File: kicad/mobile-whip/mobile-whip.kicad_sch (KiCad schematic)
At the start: 42 parts, among them J1 Conn_Coaxial, J2 USB_C_Receptacle_USB2.0, SW1 MK-12C02-G025, U1 LTC6268IS6, U2 TP4054, U3 LP2985-3.3

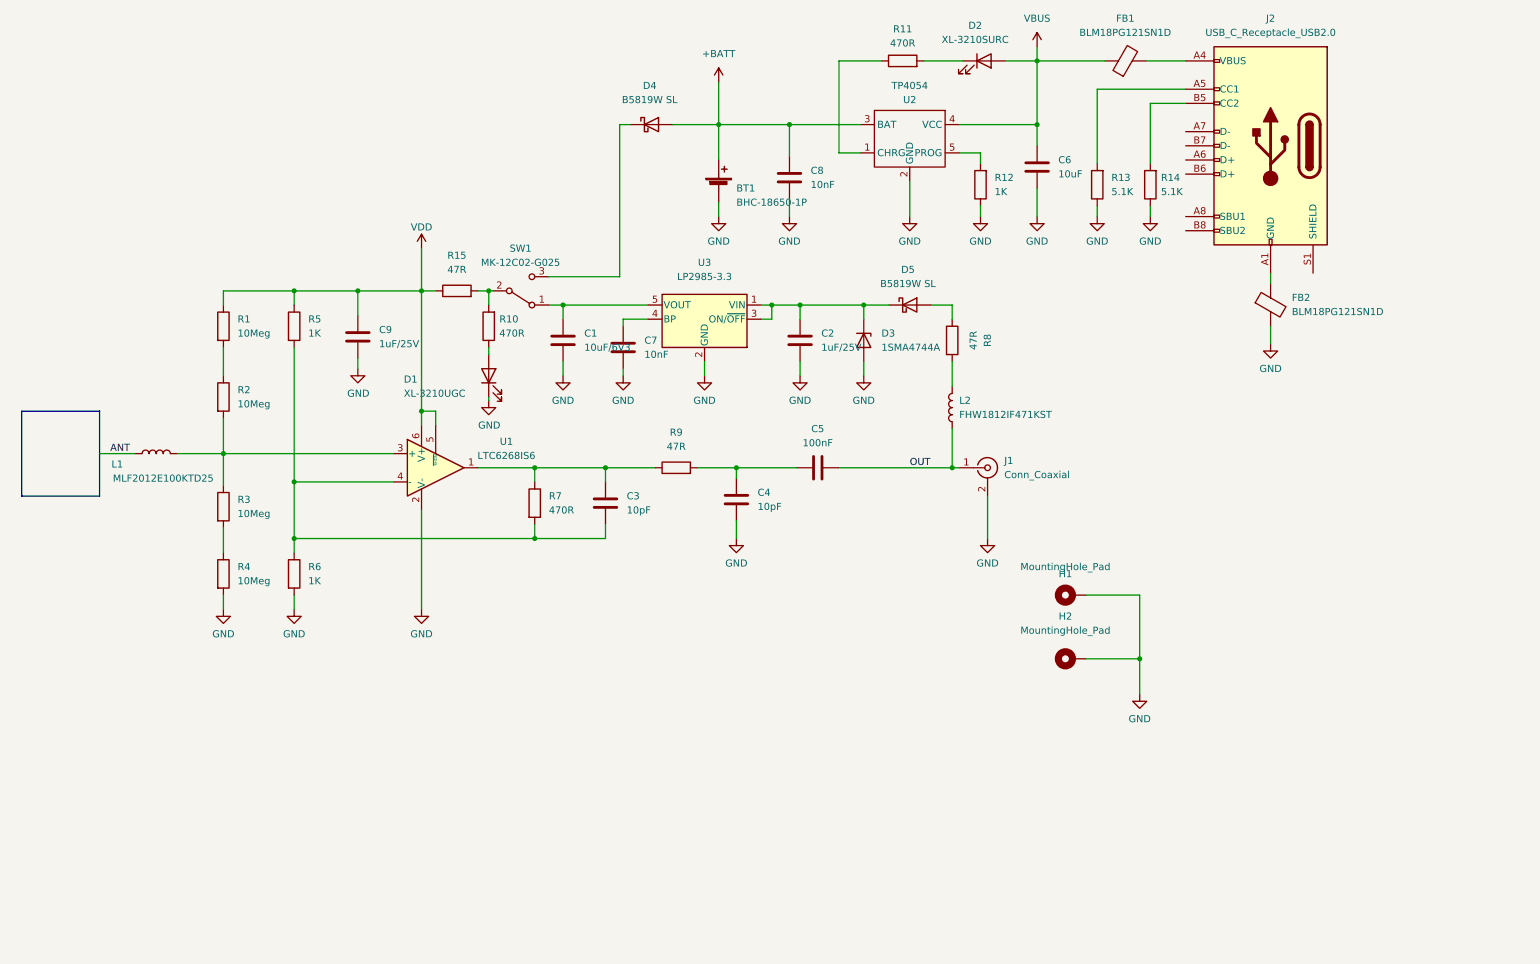
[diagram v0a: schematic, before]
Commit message: Finalize design
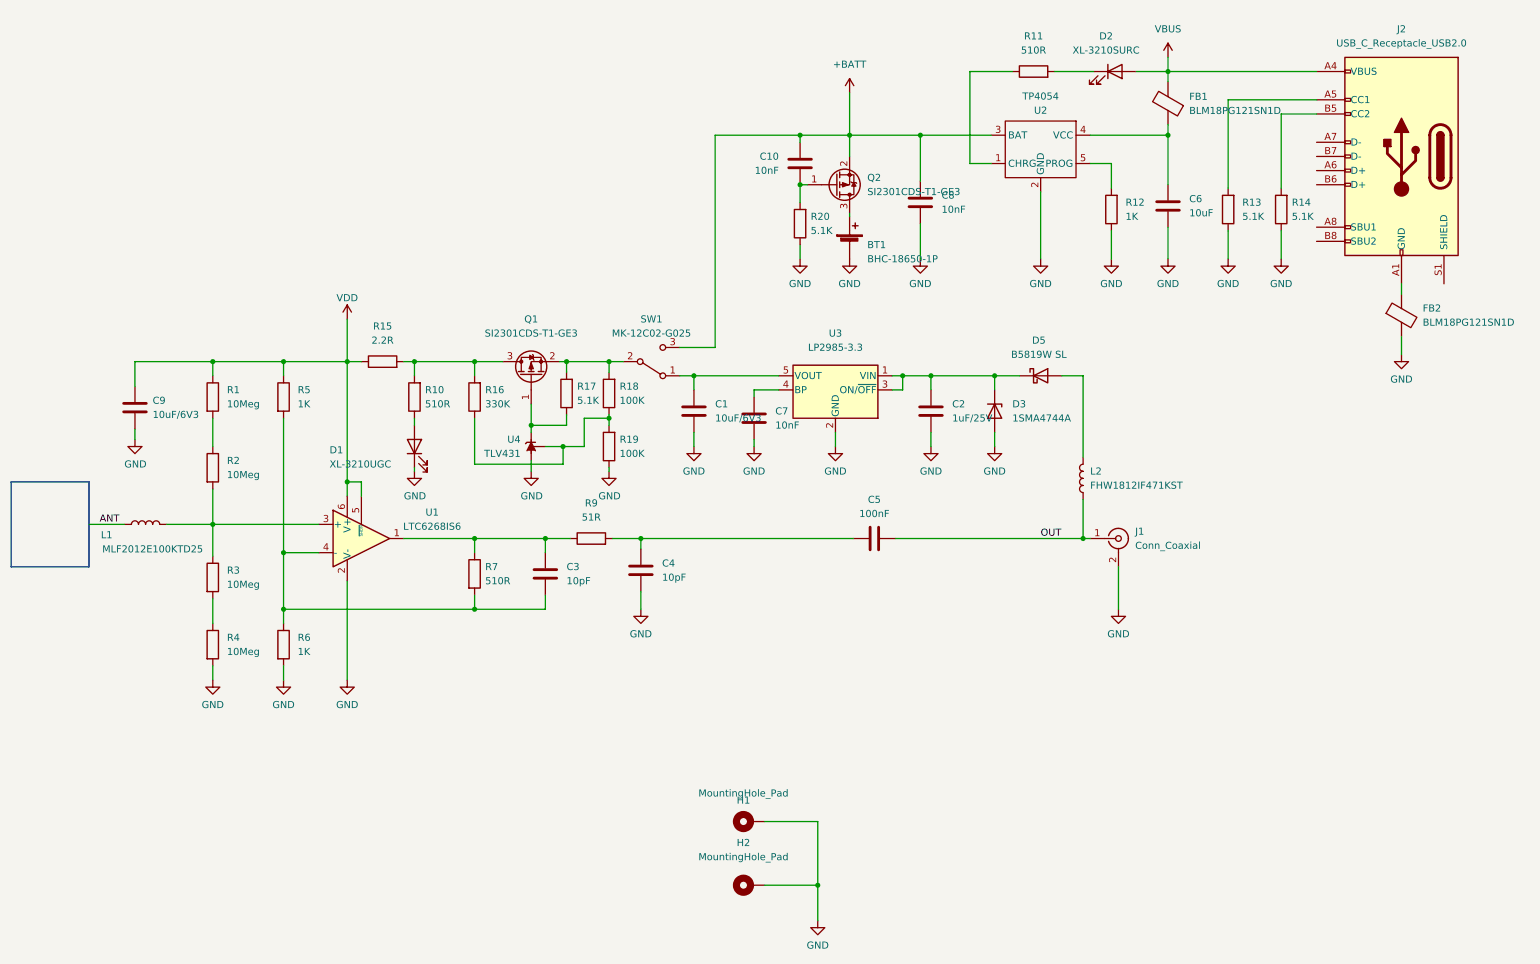
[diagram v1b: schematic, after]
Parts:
- removed D4: B5819W SL, Diode_SMD:D_SOD-123, symbol Device:D_Schottky
- removed R8: 47R, Resistor_SMD:R_1206_3216Metric, symbol Device:R
- added C10: 10nF, Capacitor_SMD:C_0805_2012Metric, symbol Device:C
- added Q1, Q2: SI2301CDS-T1-GE3, Package_TO_SOT_SMD:SOT-23, symbol Transistor_FET:AO3401A
- added R16: 330K, Resistor_SMD:R_0805_2012Metric, symbol Device:R
- added R17, R20: 5.1K, Resistor_SMD:R_0805_2012Metric, symbol Device:R
- added R18, R19: 100K, Resistor_SMD:R_0805_2012Metric, symbol Device:R
- added U4: TLV431, Package_TO_SOT_SMD:SOT-23, symbol Reference_Voltage:TL431DBZ
- C9: value 1uF/25V -> 10uF/6V3
- R10, R11, R7: value 470R -> 510R
- R15: value 47R -> 2.2R
- R9: value 47R -> 51R
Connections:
- net +BATT: now also SW1.3 (C), C10.2, Q2.2 (S); no longer BT1.1 (+)
- net GND: now also R19.1, R20.1, U4.3 (A)
- net VBUS: now also FB1.2, J2.A4 (VBUS), J2.A9 (VBUS), J2.B4 (VBUS), J2.B9 (VBUS); no longer C6.1, FB1.1, U2.4 (VCC)
- net at R10.2, R15.2: now also Q1.3 (D), R16.2; no longer SW1.2 (B)
- net at D5.2 (A): now also L2.2
- new net: R16.1, R18.1, R19.2, U4.2 (REF)
- new net: Q1.2 (S), R17.2, R18.2, SW1.2 (B)
- new net: C6.1, FB1.1, U2.4 (VCC)
- new net: BT1.1 (+), Q2.3 (D)
- new net: Q1.1 (G), R17.1, U4.1 (K)
- new net: C10.1, Q2.1 (G), R20.2
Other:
- moved on the sheet: BT1, C1, C2, C3, C4, C5, C6, C7, C8, C9, D1, D2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
